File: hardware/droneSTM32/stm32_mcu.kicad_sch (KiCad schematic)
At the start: 33 parts, among them U101 STM32F103R8T6

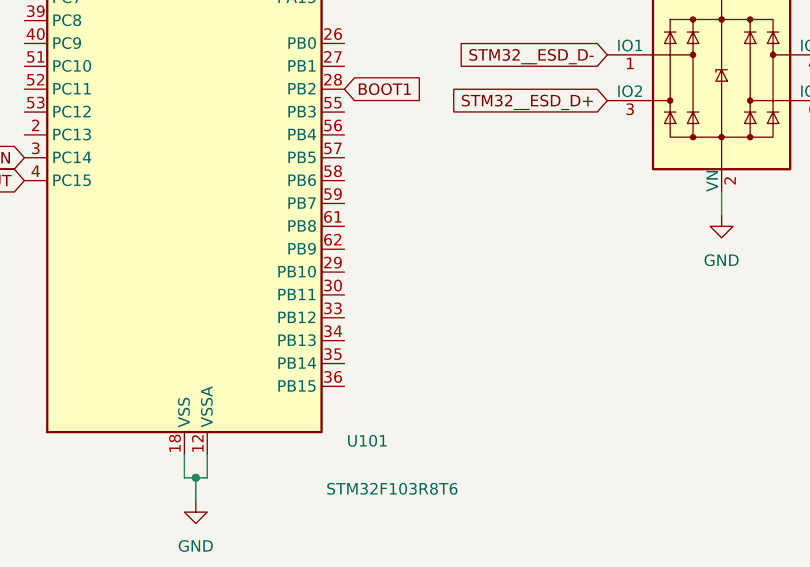
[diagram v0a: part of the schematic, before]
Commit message: commit mpu6050 update
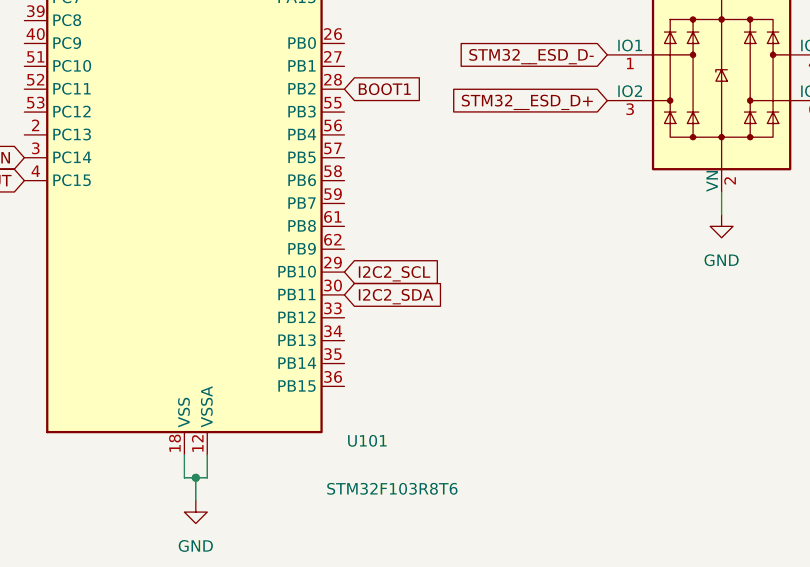
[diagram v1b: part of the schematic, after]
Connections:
- net I2C2_SCL: now reaches U101.29 (PB10)
- net I2C2_SDA: now reaches U101.30 (PB11)
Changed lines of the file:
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@@
+		)
+	)
+	(global_label "I2C2_SDA"
+		(shape input)
+		(at 172.72 128.27 0)
+		(fields_autoplaced yes)
+		(effects
+			(font
+				(size 1.27 1.27)
+			)
+			(justify left)
+		)
+		(property "Intersheetrefs" "${INTERSHEET_REFS}"
+			(at 184.5347 128.27 0)
+			(hide yes)
+			(show_name no)
+			(do_not_autoplace no)
+			(effects
+				(font
+					(size 1.27 1.27)
+				)
+				(justify left)
+			)
 		)
 	)
@@
 			)
 		)
+	)
+	(global_label "I2C2_SCL"
+		(shape input)
+		(at 172.72 125.73 0)
+		(fields_autoplaced yes)
+		(effects
+			(font
+				(size 1.27 1.27)
+			)
+			(justify left)
+		)
+		(property "Intersheetrefs" "${INTERSHEET_REFS}"
+			(at 184.4742 125.73 0)
+			(hide yes)
+			(show_name no)
+			(do_not_autoplace no)
+			(effects
+				(font
+					(size 1.27 1.27)
+				)
+				(justify left)
+			)
+		)
